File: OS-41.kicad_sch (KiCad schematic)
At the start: 58 parts, among them IC1 SI4432-B1-FMR, J1 Conn_Coaxial, J2 Conn_01x02_Pin, J3 Conn_01x04_Pin, J4 Conn_01x02_Pin, J5 Conn_01x02_Pin, J6 Conn_01x02_Pin, J7 Conn_01x02_Pin, SW1 TS-1187A-B-A-B, SW2 TS-1187A-B-A-B, SW3 TS-1187A-B-A-B, U1 ESP-12F, U2 ATGM336H-5N31, U3 DS18B20, U4 DS18B20, U5 MCP1640x-xCHY, U6 TLV62569DBVR, U7 GPS1003, X1 SMD-3225_4P 30.000MHZ 10PF

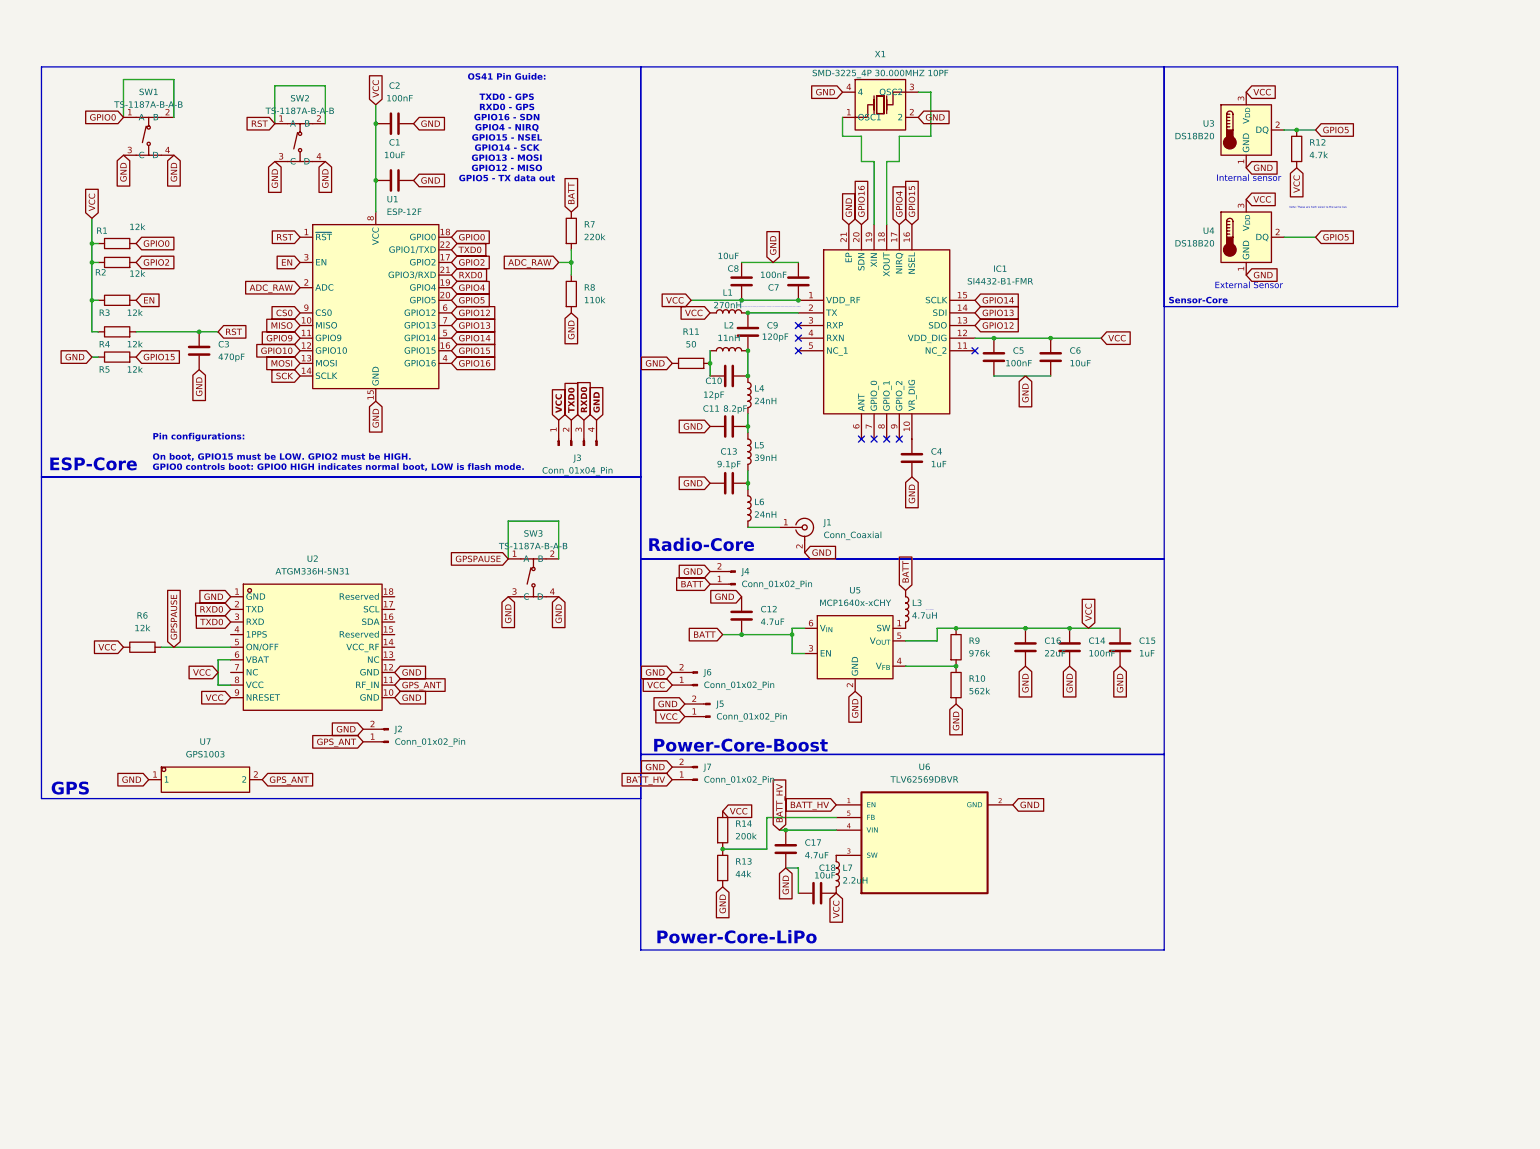
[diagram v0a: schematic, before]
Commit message: Major board revamp!
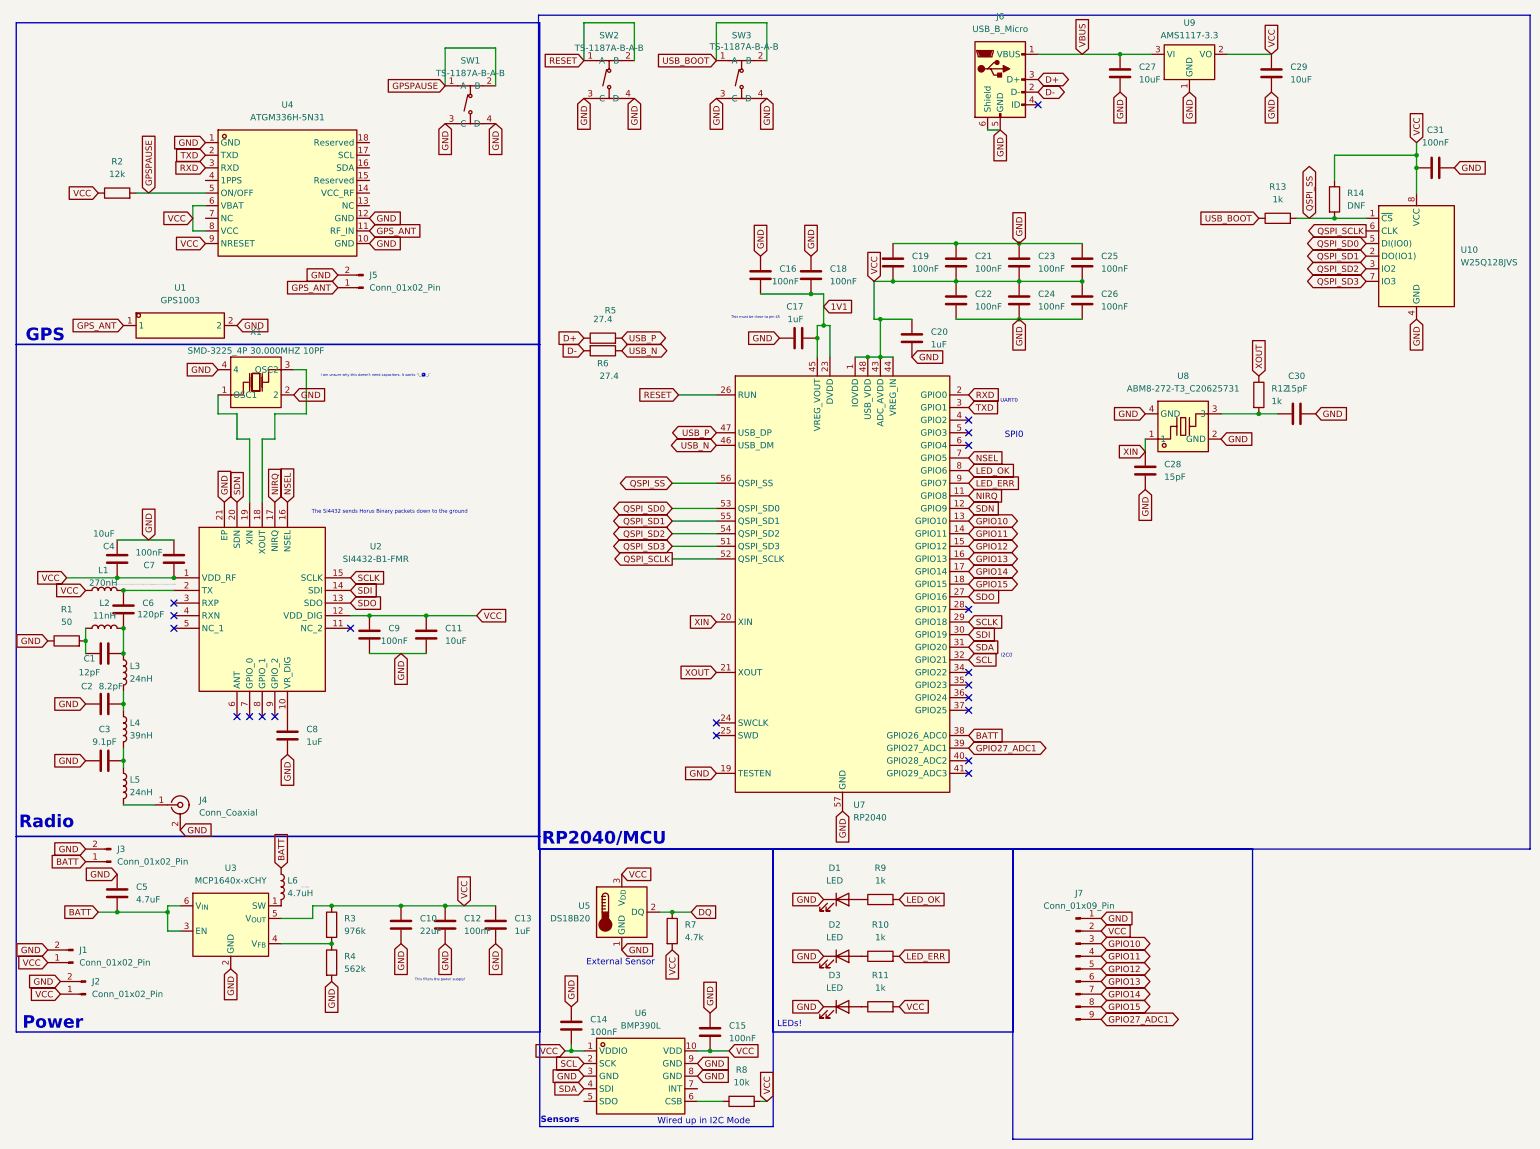
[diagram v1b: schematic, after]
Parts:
- removed C1: 10uF, Capacitor_SMD:C_0603_1608Metric_Pad1.08x0.95mm_HandSolder, symbol Device:C
- removed C2: 100nF, Capacitor_SMD:C_0603_1608Metric_Pad1.08x0.95mm_HandSolder, symbol Device:C
- removed C3: 470pF, Capacitor_SMD:C_0603_1608Metric_Pad1.08x0.95mm_HandSolder, symbol Device:C
- removed J3: Conn_01x04_Pin, Connector_PinSocket_2.54mm:PinSocket_1x04_P2.54mm_Vertical, symbol Connector:Conn_01x04_Pin
- removed J7: Conn_01x02_Pin, Connector_PinSocket_2.54mm:PinSocket_1x02_P2.54mm_Vertical, symbol Connector:Conn_01x02_Pin
- removed L7: 2.2uH, Inductor_SMD:L_0603_1608Metric_Pad1.05x0.95mm_HandSolder, symbol Device:L
- removed R1, R2, R3, R4: 12k, Resistor_SMD:R_0603_1608Metric_Pad0.98x0.95mm_HandSolder, symbol Device:R
- removed R7: 220k, Resistor_SMD:R_0603_1608Metric_Pad0.98x0.95mm_HandSolder, symbol Device:R
- removed SW1: TS-1187A-B-A-B, libsos41:SW-SMD_4P-L5.1-W5.1-P3.70-LS6.5-TL-2, symbol libs:TS-1187A-B-A-B
- removed U1: ESP-12F, RF_Module:ESP-12E, symbol RF_Module:ESP-12F
- removed U4: DS18B20, Package_TO_SOT_THT:TO-92_Inline, symbol Sensor_Temperature:DS18B20
- removed U6: TLV62569DBVR, centdir:SOT95P280X145-5N, symbol downconv:TLV62569DBVR
- added C14, C15, C16, C19, C21, C22, C23, C24, C25, C26, C31: 100nF, Capacitor_SMD:C_0603_1608Metric_Pad1.08x0.95mm_HandSolder, symbol Device:C
- added C20: 1uF, Capacitor_SMD:C_0603_1608Metric_Pad1.08x0.95mm_HandSolder, symbol Device:C
- added C27, C29: 10uF, Capacitor_SMD:C_0603_1608Metric_Pad1.08x0.95mm_HandSolder, symbol Device:C
- added C28, C30: 15pF, Capacitor_SMD:C_0603_1608Metric_Pad1.08x0.95mm_HandSolder, symbol Device:C
- added D1, D2, D3: LED, LED_SMD:LED_0805_2012Metric_Pad1.15x1.40mm_HandSolder, symbol Device:LED
- added J6: USB_B_Micro, libsos41:MICRO-USB-SMD_MICRO-USB-18, symbol Connector:USB_B_Micro
- added J7: Conn_01x09_Pin, Connector_PinSocket_2.54mm:PinSocket_1x09_P2.54mm_Vertical, symbol Connector:Conn_01x09_Pin
- added R10, R11, R12, R9: 1k, Resistor_SMD:R_0603_1608Metric_Pad0.98x0.95mm_HandSolder, symbol Device:R
- added R6: 27.4, Resistor_SMD:R_0603_1608Metric_Pad0.98x0.95mm_HandSolder, symbol Device:R
- added SW3: TS-1187A-B-A-B, libsos41:SW-SMD_4P-L5.1-W5.1-P3.70-LS6.5-TL-2, symbol libs:TS-1187A-B-A-B
- added U10: W25Q128JVS, Package_SO:SOIC-8_5.23x5.23mm_P1.27mm, symbol Memory_Flash:W25Q128JVS
- added U6: BMP390L, libsos41:LGA-10_L2.0-W2.0-P0.50-TL_BMP390L, symbol libs:BMP390L
- added U7: RP2040, Package_DFN_QFN:QFN-56-1EP_7x7mm_P0.4mm_EP3.2x3.2mm, symbol MCU_RaspberryPi:RP2040
- added U8: ABM8-272-T3_C20625731, libsos41:CRYSTAL-SMD_4P-L3.2-W2.5-BL, symbol libs:ABM8-272-T3_C20625731
- added U9: AMS1117-3.3, Package_TO_SOT_SMD:SOT-223-3_TabPin2, symbol Regulator_Linear:AMS1117-3.3
- C17: value 4.7uF -> 1uF
- C18: value 10uF -> 100nF
- R13: value 44k -> 1k
- R14: value 200k -> DNF
- R5: value 12k -> 27.4
- R8: value 110k -> 10k
- renumbered C10 to C1, C16 to C10, C6 to C11, C14 to C12, C15 to C13, C11 to C2, C13 to C3, C8 to C4, C12 to C5, C9 to C6, C4 to C8, C5 to C9, J6 to J1, J5 to J2, J4 to J3, J1 to J4, J2 to J5, L4 to L3, L5 to L4, L6 to L5, L3 to L6, R11 to R1, R6 to R2, R9 to R3, R10 to R4, R12 to R7, SW3 to SW1, U7 to U1, IC1 to U2, U5 to U3, U2 to U4, U3 to U5
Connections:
- net BATT_HV is gone; now on net GND: C17.1
- net BATT: now also U7.38 (GPIO26_ADC0)
- net GND: now also U1.2, C14.1, C15.1, C16.1, C19.1, C20.2, C21.1, C22.2, C23.1, C24.2, C25.1, C26.2, C27.2, C28.2, C29.2, C30.2, C31.2, D1.1 (K), D2.1 (K), D3.1 (K), J6.5 (GND), J6.6 (Shield), J7.1 (Pin_1), SW3.3 (C), SW3.4 (D), U10.4 (GND), U6.3 (GND), U6.8 (GND), U6.9 (GND), U7.19 (TESTEN), U7.57 (GND), U8.2 (GND), U8.4 (GND), U9.1 (GND); no longer C17.2, R13.2, R5.1, R8.2, U1.1
- net GPIO10: now also J7.3 (Pin_3), U7.13 (GPIO10)
- net GPIO12: now also J7.5 (Pin_5), U7.15 (GPIO12); no longer U2.13 (SDO)
- net GPIO13: now also J7.6 (Pin_6), U7.16 (GPIO13); no longer U2.14 (SDI)
- net GPIO14: now also J7.7 (Pin_7), U7.17 (GPIO14); no longer U2.15 (SCLK)
- net GPIO15: now also J7.8 (Pin_8), U7.18 (GPIO15); no longer R5.2, U2.16 (NSEL)
- net GPS_ANT: now also U1.1; no longer U1.2
- net VCC: now also R8.2, C14.2, C15.2, C19.2, C20.1, C21.2, C22.1, C23.2, C24.1, C25.2, C26.1, C29.1, C31.1, J7.2 (Pin_2), R11.2, U10.8 (VCC), U6.1 (VDDIO), U6.10 (VDD), U7.1 (IOVDD), U7.10 (IOVDD), U7.22 (IOVDD), U7.33 (IOVDD), U7.42 (IOVDD), U7.43 (ADC_AVDD), U7.44 (VREG_IN), U7.48 (USB_VDD), U7.49 (IOVDD), U9.2 (VO); no longer C18.2
- net QSPI_SS: now reaches R14.2
- net QSPI_SS: now also R13.2, U10.1 (~{CS}), U7.56 (QSPI_SS); no longer R13.1
- net ADC_RAW: no longer names the net of R8.1
- net ADC_RAW: now also U6.6 (CSB)
- net GPIO16 renamed SDN
- net SDN: now also U7.12 (GPIO9)
- net GPIO4 renamed NIRQ
- net NIRQ: now also U7.11 (GPIO8)
- net GPIO5 renamed DQ
- net RST renamed RESET
- net RESET: now also U7.26 (RUN)
- net RXD0 renamed TXD
- net TXD: now also U7.3 (GPIO1)
- net TXD0 renamed RXD
- net RXD: now also U7.2 (GPIO0)
- new net: D1.2 (A), R9.1
- new net: C30.1, R12.2, U8.3
- new net: D2.2 (A), R10.1
- new net: D3.2 (A), R11.1
- new net 1V1: C16.2, C17.2, C18.2, U7.23 (DVDD), U7.45 (VREG_VOUT), U7.50 (DVDD)
- new net D+: J6.3 (D+), R5.1
- new net D-: J6.2 (D-), R6.2
- new net GPIO11: J7.4 (Pin_4), U7.14 (GPIO11)
- new net GPIO27_ADC1: J7.9 (Pin_9), U7.39 (GPIO27_ADC1)
- new net LED_ERR: R10.2, U7.9 (GPIO7)
- new net LED_OK: R9.2, U7.8 (GPIO6)
- new net NSEL: U2.16 (NSEL), U7.7 (GPIO5)
- new net QSPI_SCLK: U10.6 (CLK), U7.52 (QSPI_SCLK)
- new net QSPI_SD0: U10.5 (DI(IO0)), U7.53 (QSPI_SD0)
- new net QSPI_SD1: U10.2 (DO(IO1)), U7.55 (QSPI_SD1)
- new net QSPI_SD2: U10.3 (IO2), U7.54 (QSPI_SD2)
- new net QSPI_SD3: U10.7 (IO3), U7.51 (QSPI_SD3)
- new net SCL: U6.2 (SCK), U7.32 (GPIO21)
- new net SCLK: U2.15 (SCLK), U7.29 (GPIO18)
- new net SDA: U6.4 (SDI), U7.31 (GPIO20)
- new net SDI: U2.14 (SDI), U7.30 (GPIO19)
- new net SDO: U2.13 (SDO), U7.27 (GPIO16)
- new net USB_BOOT: R13.1, SW3.1 (A), SW3.2 (B)
- new net USB_N: R6.1, U7.46 (USB_DM)
- new net USB_P: R5.2, U7.47 (USB_DP)
- new net VBUS: C27.1, J6.1 (VBUS), U9.3 (VI)
- new net XIN: C28.1, U7.20 (XIN), U8.1
- new net XOUT: R12.1, U7.21 (XOUT)
- no-connect marks 8 -> 21
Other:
- note added: "I am unsure why this doesn't need capacitors. It works ¯\_(ツ)_/¯"
- note added: "I2C0"
- note added: "LEDs!"
- note added: "Power"
- note added: "RP2040/MCU"
- note added: "Radio"
- note added: "SPI0"
- note added: "Sensors"
- note added: "The Si4432 sends Horus Binary packets down to the ground"
- note added: "This filters the power supply!"
- note added: "This must be close to pin 45"
- note added: "UART0"
- note added: "Wired up in I2C Mode"
- note removed: "ESP-Core"
- note removed: "Internal sensor"
- note removed: "Note: These are both wired to the same bus"
- note removed: "OS41 Pin Guide: TXD0 - GPS RXD0 - GPS GPIO16 - SDN GPIO4 - NIRQ GPIO15 - NSEL GPIO14 - SCK GPIO13 - MOSI GPIO12 - MISO GPIO5 - TX data out"
- note removed: "Pin configurations: On boot, GPIO15 must be LOW. GPIO2 must be HIGH. GPIO0 controls boot: GPIO0 HIGH indicates normal boot, LOW is flash mode."
- note removed: "Power-Core-Boost"
- note removed: "Power-Core-LiPo"
- note removed: "Radio-Core"
- note removed: "Sensor-Core"
- moved on the sheet: C1, C10, C11, C12, C13, C2, C3, C4, C5, C6, C7, C8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
